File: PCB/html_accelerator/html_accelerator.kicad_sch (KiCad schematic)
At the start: 0 parts

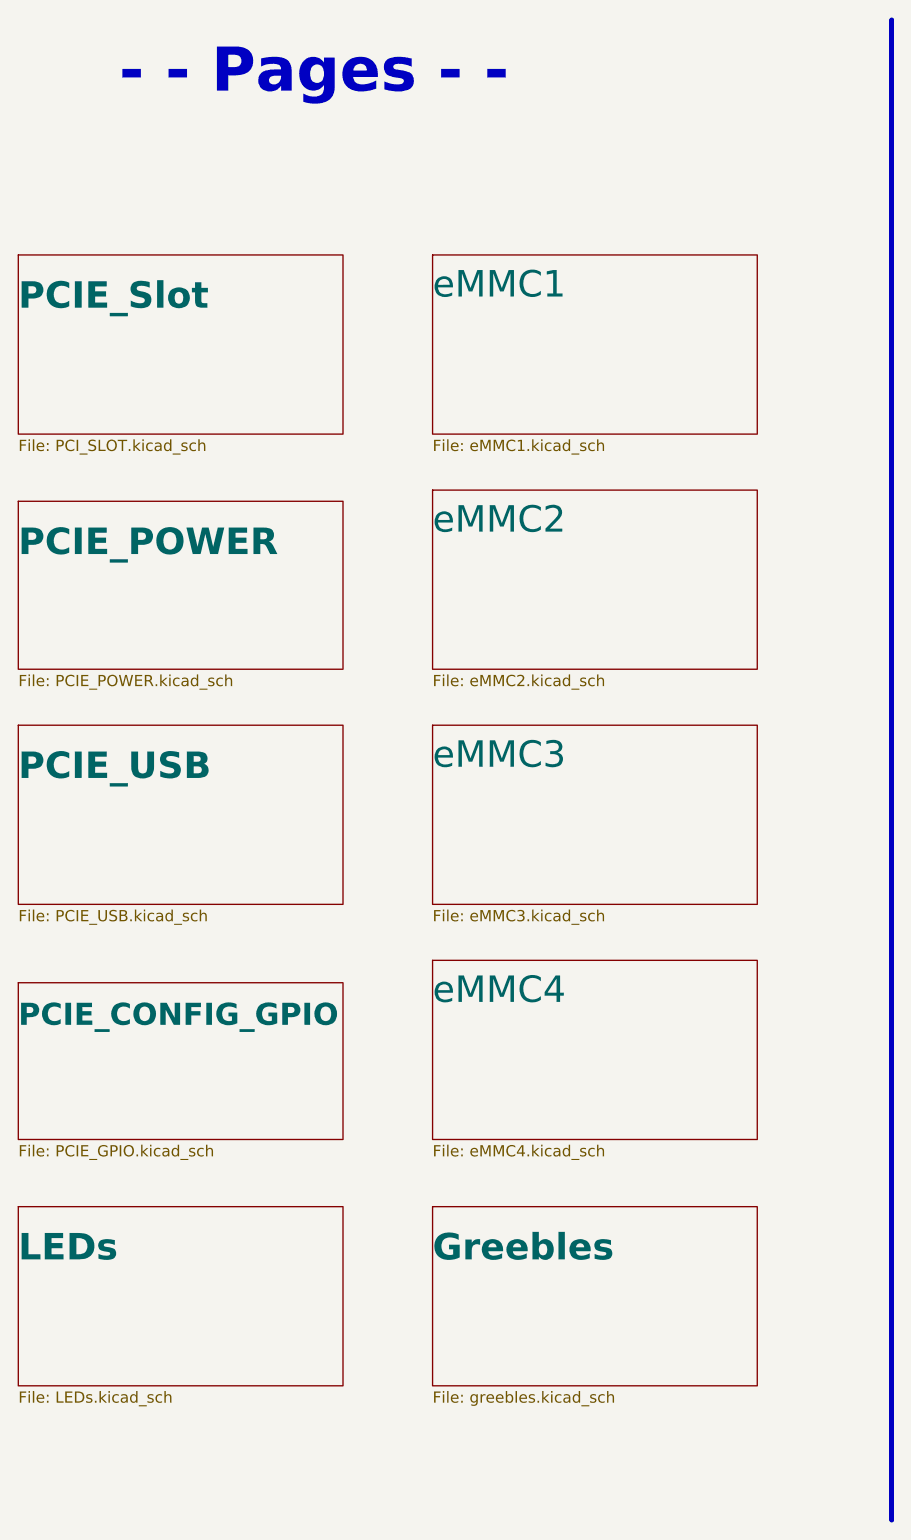
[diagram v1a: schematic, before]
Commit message: gerbers and readme updates
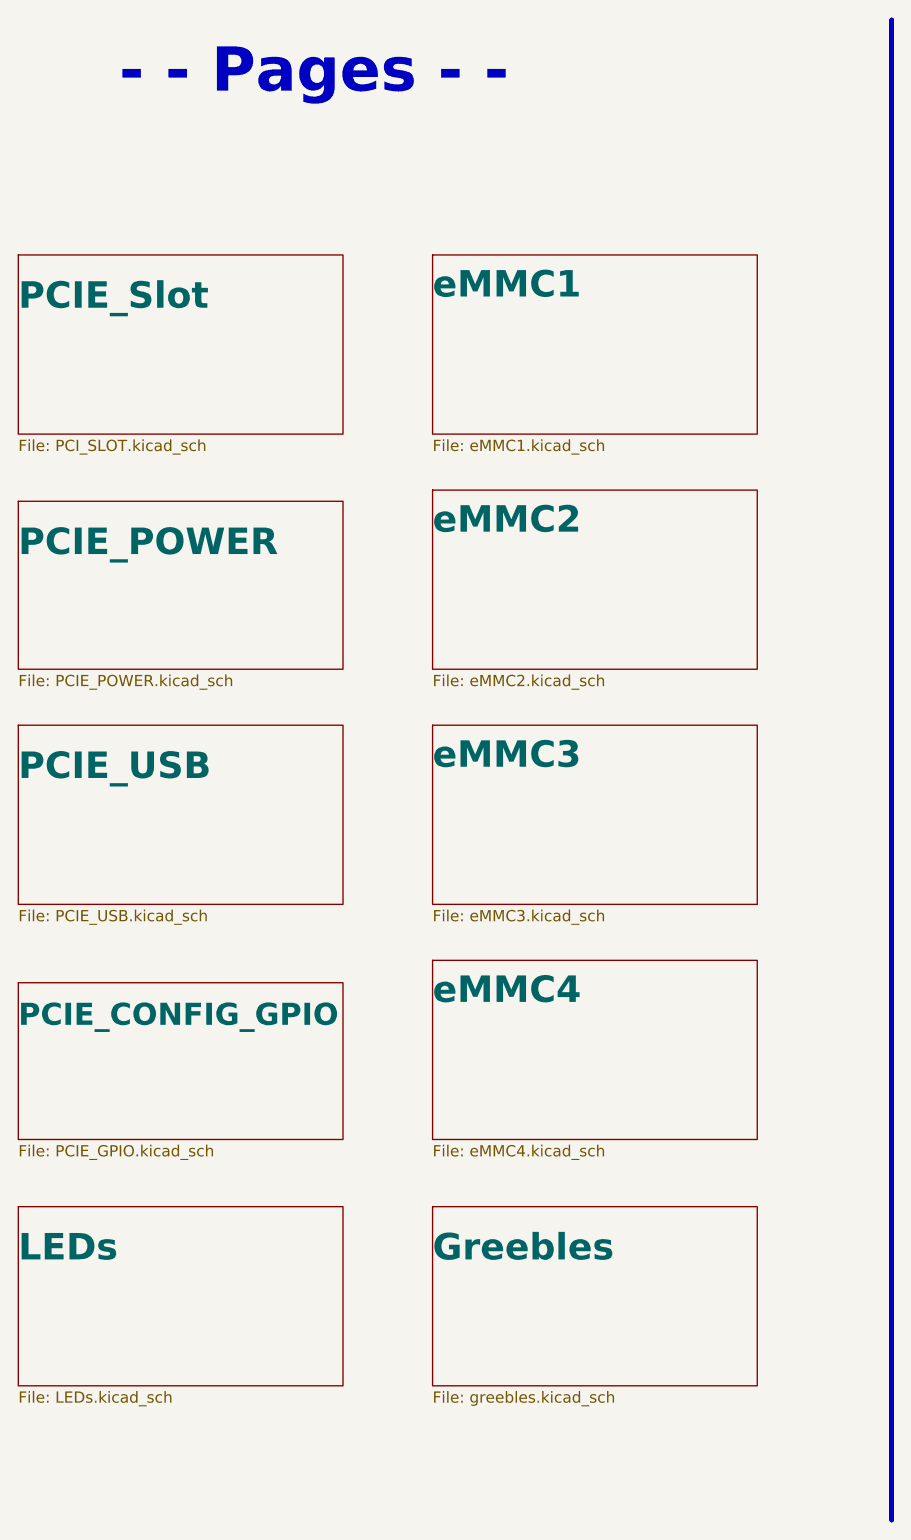
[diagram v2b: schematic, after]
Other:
- company: (none) -> Spencer K
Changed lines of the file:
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@@
 	(title_block
 		(title "HTML Accelerator")
-		(date "2024-10-07")
+		(date "2026-04-25")
 		(rev "1.0")
+		(company "Spencer K")
+		(comment 1 "https://github.com/akaStanley/HTML_Accelerator")
 	)
 	(rectangle
@@
 			(project "html_accelerator"
 				(path "/12b3a7c9-141f-40ba-9ebb-094b58bfa6c7"
-					(page "7")
+					(page "15")
 				)
 			)
@@
 				(font
 					(size 3 3)
+					(thickness 0.6)
+					(bold yes)
 				)
 				(justify left bottom)
@@
 				(font
 					(size 3 3)
+					(thickness 0.6)
+					(bold yes)
 				)
 				(justify left bottom)
@@
 				(font
 					(size 3 3)
+					(thickness 0.6)
+					(bold yes)
 				)
 				(justify left bottom)
@@
 				(font
 					(size 3 3)
+					(thickness 0.6)
+					(bold yes)
 				)
 				(justify left bottom)
